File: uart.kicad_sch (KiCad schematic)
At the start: 0 parts

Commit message: added usbc power supply
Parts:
- added U7: MCP2200-I-SO, Package_SO:SOIC-20W_7.5x12.8mm_P1.27mm, symbol Interface_USB:MCP2200-I-SO
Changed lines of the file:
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@@
 	(generator_version "8.0")
 	(paper "A4")
+	(symbol
+		(lib_id "Interface_USB:MCP2200-I-SO")
+		(at 137.16 86.36 0)
+		(unit 1)
+		(exclude_from_sim no)
+		(in_bom yes)
+		(on_board yes)
+		(dnp no)
+		(fields_autoplaced yes)
+		(property "Reference" "U7"
+			(at 139.3541 106.68 0)
+			(effects
+				(font
+					(size 1.27 1.27)
+				)
+				(justify left)
+			)
+		)
+		(property "Value" "MCP2200-I-SO"
+			(at 139.3541 109.22 0)
+			(effects
+				(font
+					(size 1.27 1.27)
+				)
+				(justify left)
+			)
+		)
+		(property "Footprint" "Package_SO:SOIC-20W_7.5x12.8mm_P1.27mm"
+			(at 137.16 115.57 0)
+			(effects
+				(font
+					(size 1.27 1.27)
+				)
+				(hide yes)
+			)
+		)
+		(property "Datasheet" "http://ww1.microchip.com/downloads/en/DeviceDoc/200022228D.pdf"
+			(at 137.16 111.76 0)
+			(effects
+				(font
+					(size 1.27 1.27)
+				)
+				(hide yes)
+			)
+		)
+		(property "Description" "USB 2.0 to UART Protocol Converter with GPIO, SOIC-20"
+			(at 137.16 86.36 0)
+			(effects
+				(font
+					(size 1.27 1.27)
+				)
+				(hide yes)
+			)
+		)
+		(pin "3"
+		)
+		(pin "1"
+		)
+		(pin "16"
+		)
+		(pin "20"
+		)
+		(pin "9"
+		)
+		(pin "12"
+		)
+		(pin "15"
+		)
+		(pin "17"
+		)
+		(pin "7"
+		)
+		(pin "10"
+		)
+		(pin "11"
+		)
+		(pin "18"
+		)
+		(pin "4"
+		)
+		(pin "2"
+		)
+		(pin "13"
+		)
+		(pin "6"
+		)
+		(pin "5"
+		)
+		(pin "8"
+		)
+		(pin "14"
+		)
+		(pin "19"
+		)
+		(instances
+			(project "stm32G0_mcu"
+				(path "/342e1e7c-839e-4cd3-a9c3-2caee679f2e5/c8fc4e98-84a4-49bd-9c1e-386db6d9dbc5"
+					(reference "U7")
+					(unit 1)
+				)
+			)
+		)
+	)
 )

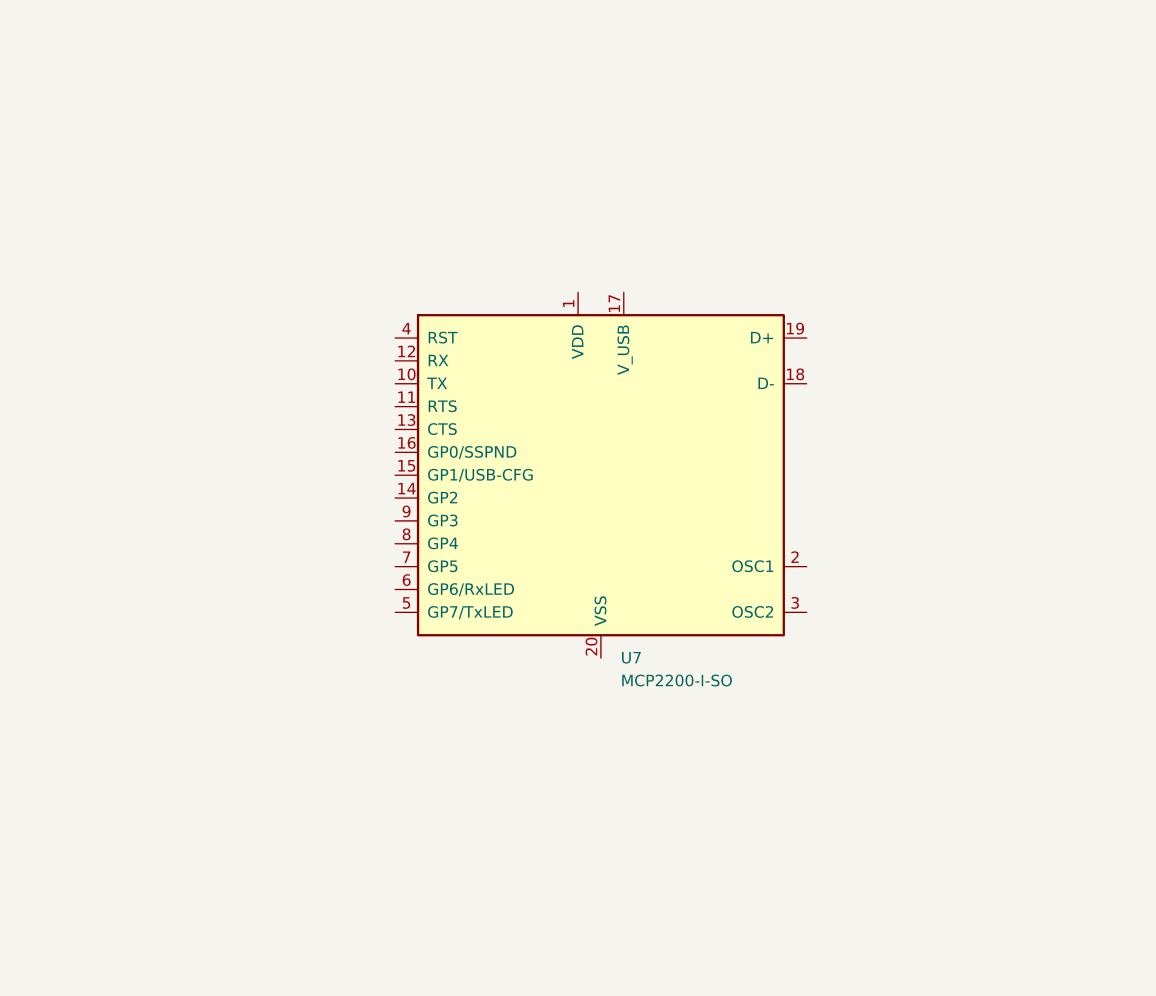
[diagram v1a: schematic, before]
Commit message: sdfdsf
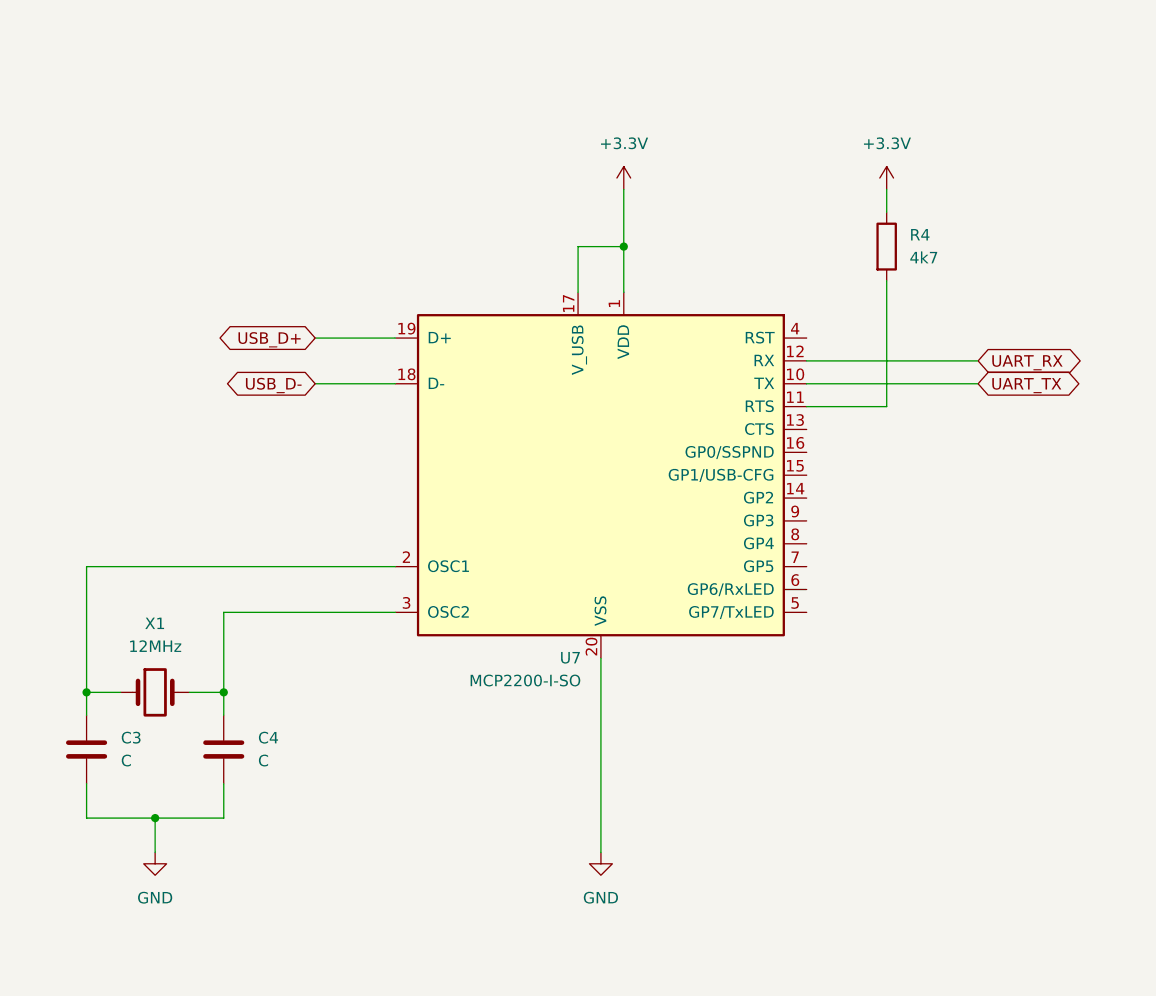
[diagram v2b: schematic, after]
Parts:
- added C3, C4: C, symbol Device:C
- added R4: 4k7, symbol Device:R
- added X1: 12MHz, symbol Device:Crystal
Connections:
- net +3.3V: now reaches U7.1 (VDD)
- net +3.3V: now also U7.17 (V_USB), R4.1
- net UART_TX: now reaches U7.10 (TX)
- net at U7.11 (RTS): now also R4.2
- net UART_RX: now reaches U7.12 (RX)
- net USB_D-: now reaches U7.18 (D-)
- net USB_D+: now reaches U7.19 (D+)
- net at U7.2 (OSC1): now also C3.1, X1.1
- net GND: now reaches U7.20 (VSS)
- net GND: now also C3.2, C4.2
- net at U7.3 (OSC2): now also C4.1, X1.2

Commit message: fsdf
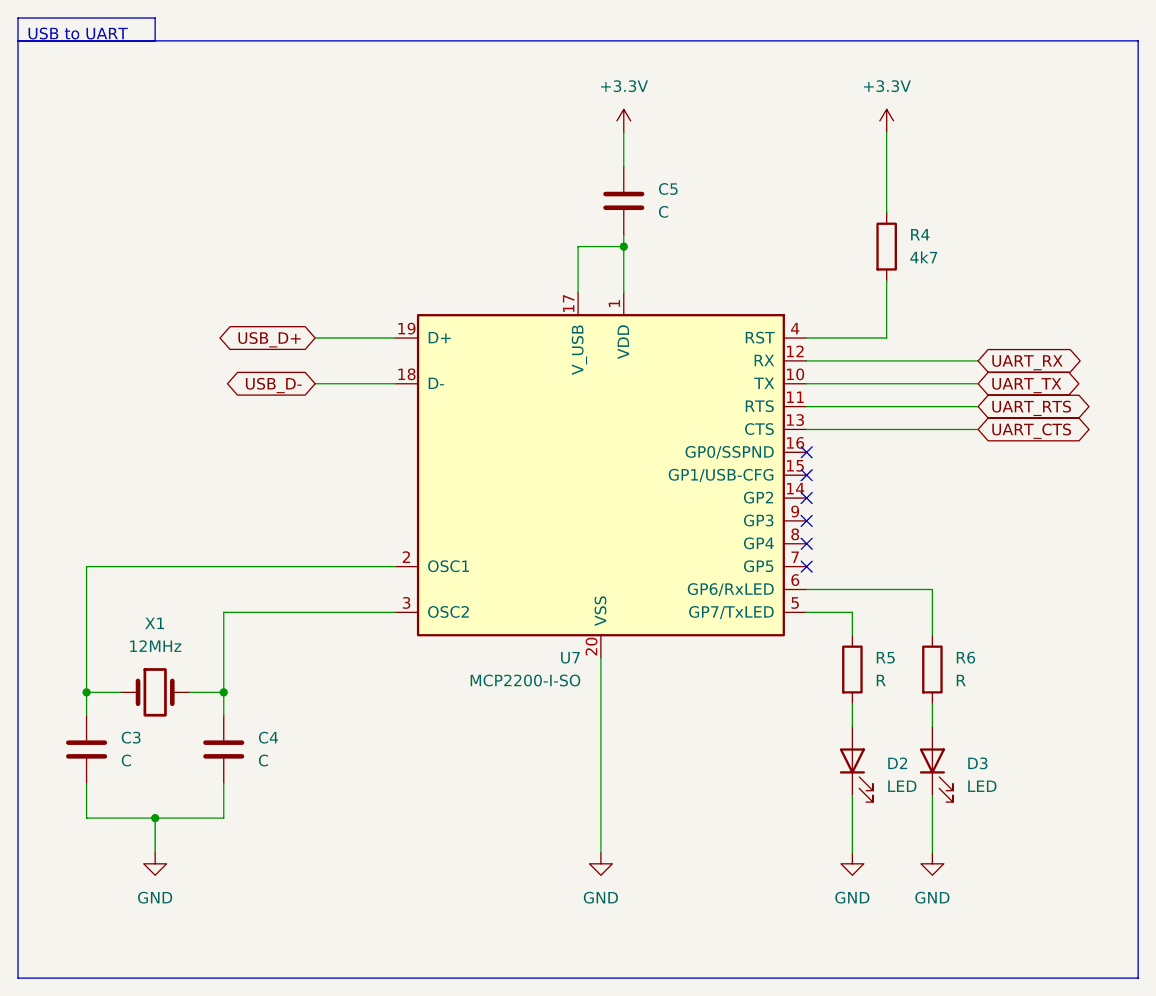
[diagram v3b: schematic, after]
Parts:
- added C5: C, symbol Device:C
- added D2, D3: LED, symbol Device:LED
- added R5, R6: R, symbol Device:R
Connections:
- net +3.3V: now also C5.1; no longer U7.1 (VDD), U7.17 (V_USB)
- net GND: now also D2.1 (K), D3.1 (K)
- net at R4.2: now also U7.4 (RST); no longer U7.11 (RTS)
- net UART_CTS: now reaches U7.13 (CTS)
- net at U7.5 (GP7/TxLED): now also R5.1
- net at U7.6 (GP6/RxLED): now also R6.1
- new net: C5.2, U7.1 (VDD), U7.17 (V_USB)
- new net: D2.2 (A), R5.2
- new net: D3.2 (A), R6.2
- new net UART_RTS: U7.11 (RTS)
- no-connect marks 0 -> 6
